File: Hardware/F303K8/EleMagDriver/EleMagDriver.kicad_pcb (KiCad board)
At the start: 2 copper layers, 104.1 x 76.2 mm, 37 parts, among them IC1 BD9E302EFJ-E2, IC2 TBD62083APG, IC3 TBD62083APG, IC4 TBD62083APG, J1 Jack-DC, J10 RelayD, J11 RelayE, J12 RelayF, J13 RelayG, J14 RelayH, J15 RelayI, J16 RelayJ, J17 Floppy_Power, J18 FloppyA, J19 Floppy_Power, J2 MotorDriverIn, J20 FloppyB, J21 Floppy_Power, J22 FloppyC, J3 MotorDriveOut, J4 SolenoidA, J5 SolenoidB, J6 StpMotor, J7 RelayA, J8 RelayB, J9 RelayC, U1 NUCLEO-F303K8

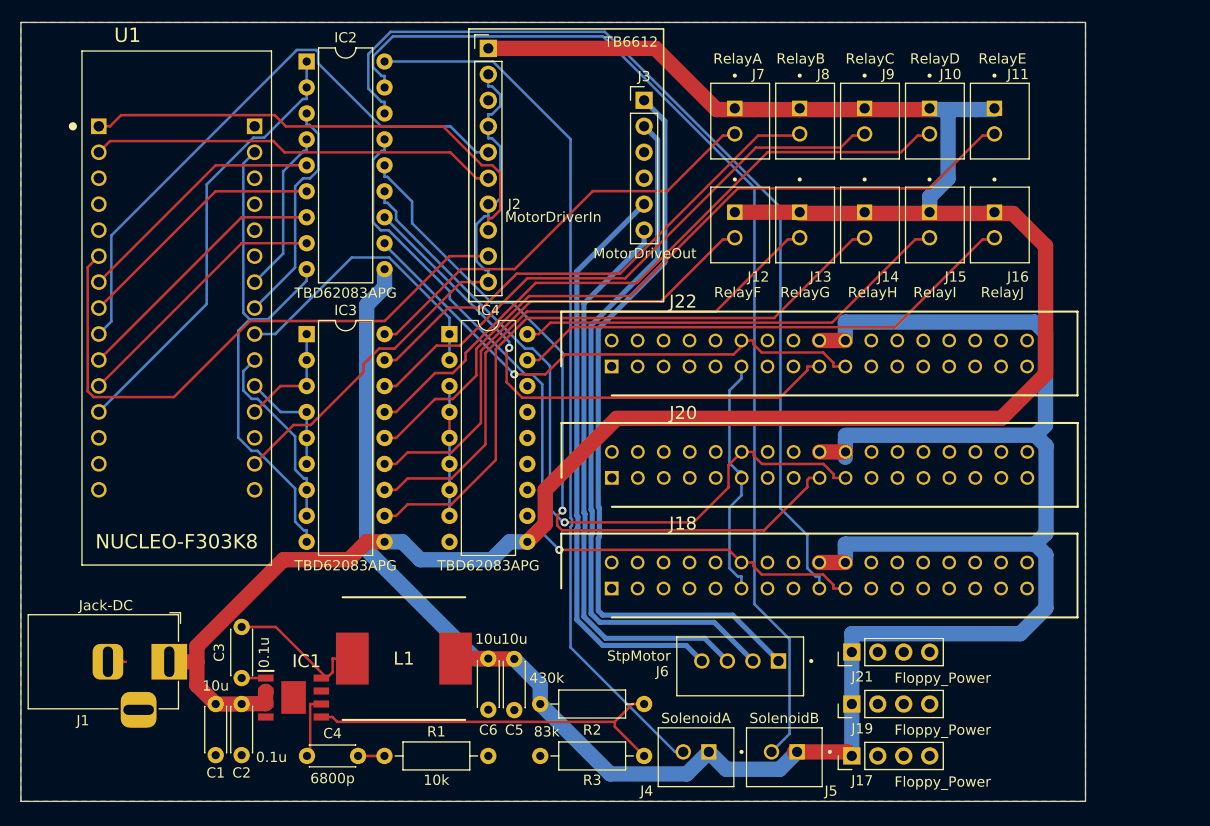
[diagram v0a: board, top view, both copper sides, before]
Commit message: edit circuit
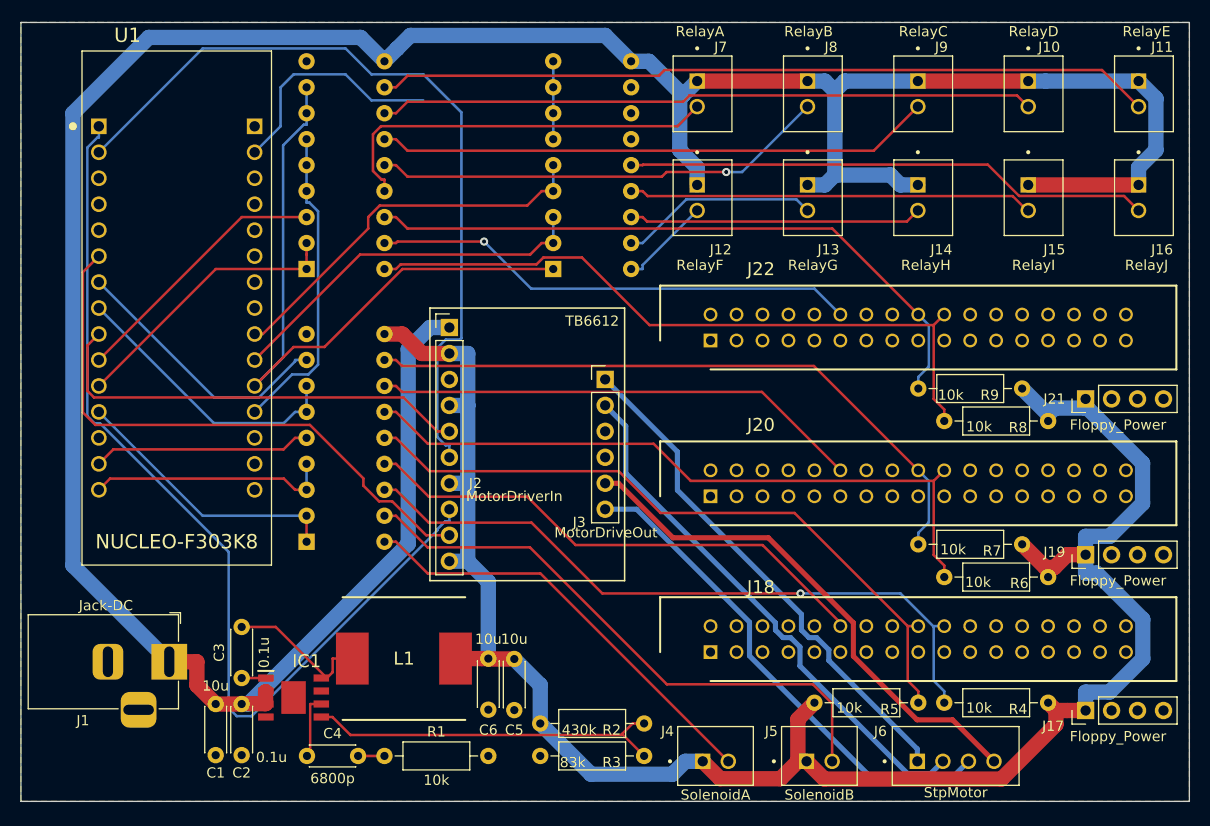
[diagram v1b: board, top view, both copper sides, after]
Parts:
- added R4: 10k, Resistor_THT:R_Axial_DIN0207_L6.3mm_D2.5mm_P10.16mm_Horizontal, F.Cu at (202.1, 117.3)
- added R5: 10k, Resistor_THT:R_Axial_DIN0207_L6.3mm_D2.5mm_P10.16mm_Horizontal, F.Cu at (179.2, 117.3)
- added R6: 10k, Resistor_THT:R_Axial_DIN0207_L6.3mm_D2.5mm_P10.16mm_Horizontal, F.Cu at (202.1, 105.1)
- added R7: 10k, Resistor_THT:R_Axial_DIN0207_L6.3mm_D2.5mm_P10.16mm_Horizontal, F.Cu at (199.5, 101.9)
- added R8: 10k, Resistor_THT:R_Axial_DIN0207_L6.3mm_D2.5mm_P10.16mm_Horizontal, F.Cu at (202.1, 89.8)
- added R9: 10k, Resistor_THT:R_Axial_DIN0207_L6.3mm_D2.5mm_P10.16mm_Horizontal, F.Cu at (199.5, 86.6)
- IC2, IC3, IC4: moved to B.Cu
- moved IC2 47.0 mm to (129.5, 101.6)
- moved J21 33.7 mm to (205.8, 87.6)
- moved J3 27.6 mm to (158.8, 85.7)
- moved J2 27.6 mm to (143.5, 80.6)
- moved J19 27.1 mm to (205.8, 102.9)
- moved J17 23.3 mm to (205.8, 118.1)
- moved J6 22.8 mm to (193.0, 122.6), turned to 0 degrees
- moved J11 14.3 mm to (211.5, 57.8)
- moved J16 14.3 mm to (211.5, 67.9)
- moved IC4 12.0 mm to (153.7, 74.9)
- moved J18 11.5 mm to (185.4, 112.4)
- moved J10 10.0 mm to (200.7, 57.8)
- moved J15 10.0 mm to (200.7, 67.9)
- moved J22 10.0 mm to (185.4, 81.9)
- moved J20 9.82 mm to (185.4, 97.2)
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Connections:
- IC2 pad 3: /Direction1 -> /Step1
- IC2 pad 5: /Step2 -> /Direction1
- IC2 pad 6: /Direction2 -> /Step2
- IC2 pad 7: /Direction3 -> /Step2
- IC2 pad 8: /Step3 -> /Direction2
- IC3 pad 1: /Relay1 -> /Step3
- IC3 pad 11: Net-(IC3-Pad11) -> Net-(J11-Pad2)
- IC3 pad 12: Net-(IC3-Pad12) -> Net-(J10-Pad2)
- IC3 pad 2: /Relay1 -> /Step3
- IC3 pad 3: /Relay1 -> /Direction3
- IC3 pad 4: /Relay2 -> /Relay1
- IC3 pad 5: /Relay2 -> /Relay1
- IC3 pad 6: /Relay2 -> /Relay1
- IC3 pad 7: /Relay3 -> /Relay2
- IC3 pad 8: /Relay3 -> /Relay2
- IC4 pad 1: /Relay4 -> /Relay2
- IC4 pad 14: unconnected-(IC4-Pad14) -> Net-(J16-Pad2)
- IC4 pad 15: unconnected-(IC4-Pad15) -> Net-(J15-Pad2)
- IC4 pad 16: unconnected-(IC4-Pad16) -> Net-(J14-Pad2)
- IC4 pad 17: Net-(IC4-Pad17) -> Net-(J13-Pad2)
- IC4 pad 18: Net-(IC4-Pad18) -> Net-(J12-Pad2)
- IC4 pad 2: /Relay4 -> /Relay3
- IC4 pad 3: GND -> /Relay3
- IC4 pad 4: GND -> /Relay4
- IC4 pad 5: GND -> /Relay4
- J10 pad 2: Net-(IC3-Pad15) -> Net-(J10-Pad2)
- J11 pad 2: Net-(IC3-Pad14) -> Net-(J11-Pad2)
- J12 pad 2: Net-(IC3-Pad13) -> Net-(J12-Pad2)
- J13 pad 2: Net-(IC3-Pad12) -> Net-(J13-Pad2)
- J14 pad 2: Net-(IC3-Pad11) -> Net-(J14-Pad2)
- J15 pad 2: Net-(IC4-Pad18) -> Net-(J15-Pad2)
- J16 pad 2: Net-(IC4-Pad17) -> Net-(J16-Pad2)
- J18 pad 11: GND -> unconnected-(J18-Pad11)
- J18 pad 17: Net-(IC2-Pad16) -> unconnected-(J18-Pad17)
- J18 pad 18: +5V -> Net-(IC2-Pad14)
- J18 pad 19: Net-(IC2-Pad15) -> unconnected-(J18-Pad19)
- J18 pad 20: +5V -> Net-(IC2-Pad16)
- J2 pad 10: +3.3V -> +5V
- J2 pad 2: +3.3V -> +5V
- J2 pad 4: +3.3V -> +5V
- J2 pad 7: +3.3V -> +5V
- J20 pad 11: GND -> unconnected-(J20-Pad11)
- J20 pad 12: Net-(IC2-Pad13) -> Net-(IC2-Pad12)
- J20 pad 17: Net-(IC2-Pad14) -> unconnected-(J20-Pad17)
- J20 pad 18: +5V -> Net-(IC2-Pad11)
- J20 pad 19: Net-(IC2-Pad13) -> unconnected-(J20-Pad19)
- J20 pad 20: +5V -> Net-(IC2-Pad13)
- J22 pad 11: GND -> unconnected-(J22-Pad11)
- J22 pad 12: Net-(IC2-Pad11) -> Net-(IC3-Pad17)
- J22 pad 17: Net-(IC2-Pad12) -> unconnected-(J22-Pad17)
- J22 pad 18: +5V -> Net-(IC3-Pad16)
- J22 pad 19: Net-(IC2-Pad11) -> unconnected-(J22-Pad19)
- J22 pad 20: +5V -> Net-(IC3-Pad18)
- J7 pad 2: Net-(IC3-Pad18) -> Net-(IC3-Pad15)
- J8 pad 2: Net-(IC3-Pad17) -> Net-(IC3-Pad14)
- J9 pad 2: Net-(IC3-Pad16) -> Net-(IC3-Pad13)
- U1 pad 3_14: unconnected-(U1-Pad3_14) -> /Direction1
- U1 pad 3_15: unconnected-(U1-Pad3_15) -> /Step1
- U1 pad 3_7: /Step2 -> /Direction2
- U1 pad 3_8: /Direction2 -> /Step2
- U1 pad 4_14: +3.3V -> unconnected-(U1-Pad4_14)
- U1 pad 4_7: /Step1 -> unconnected-(U1-Pad4_7)
- U1 pad 4_8: /Direction1 -> unconnected-(U1-Pad4_8)
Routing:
- net Net-(J11-Pad2): track 0.00 -> 76.0 mm
- net Net-(IC3-Pad11): track 64.5 -> 0.00 mm
- net Net-(J10-Pad2): track 0.00 -> 64.1 mm
- net +12V: track 219.9 -> 283.0 mm
- net GND: track 90.1 -> 30.6 mm
- net Net-(IC3-Pad12): track 56.0 -> 0.00 mm
- net +3.3V: track 55.5 -> 0.00 mm
- net /Relay2: track 11.2 -> 65.4 mm
- net Net-(J16-Pad2): track 0.00 -> 51.5 mm
- net Net-(IC4-Pad17): track 50.6 -> 0.00 mm
- net Net-(IC2-Pad17): track 105.3 -> 57.1 mm
- net /Stp_A: track 48.4 -> 94.6 mm
- net Net-(IC2-Pad18): track 86.4 -> 42.5 mm
- net Net-(IC4-Pad18): track 43.2 -> 0.00 mm
- net Net-(J15-Pad2): track 0.00 -> 39.6 mm
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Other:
- board size 104.1 x 76.2 mm -> 114.3 x 76.2 mm
